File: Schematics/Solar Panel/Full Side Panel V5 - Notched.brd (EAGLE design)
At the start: 50 x 50 mm, 24 parts

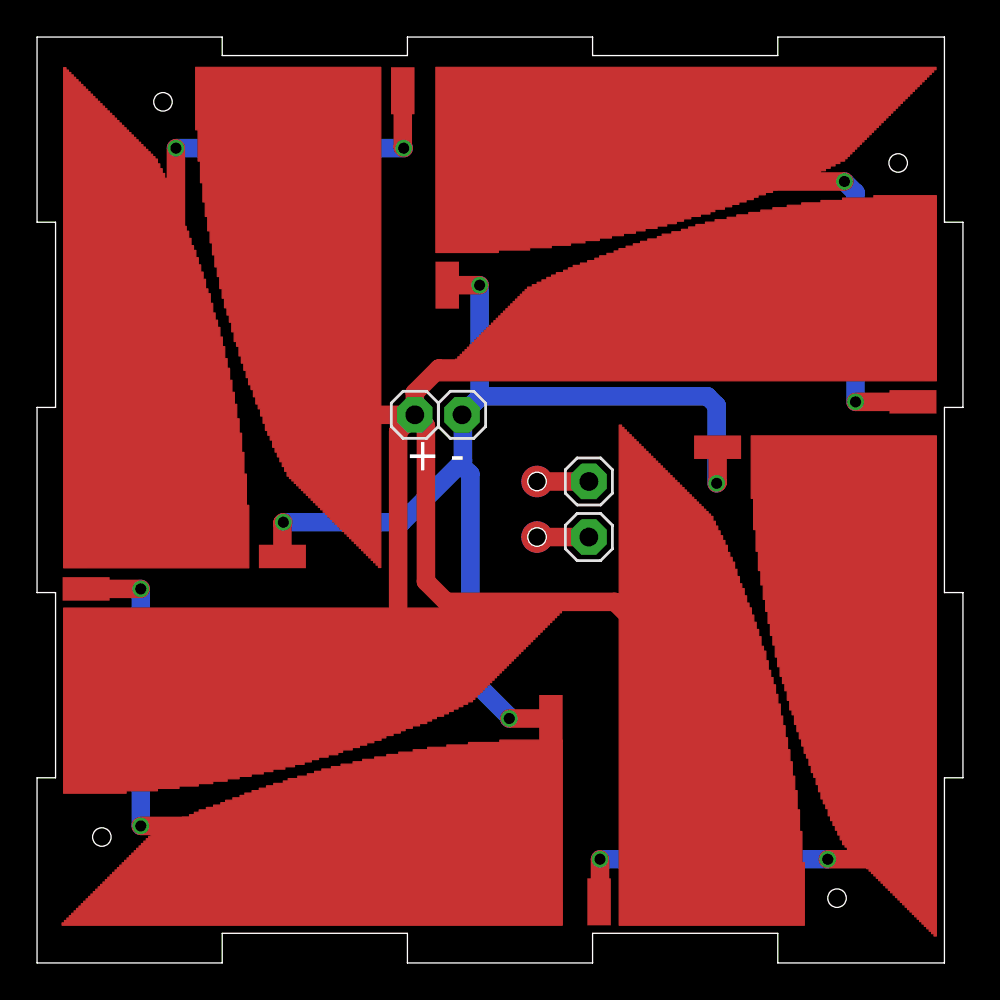
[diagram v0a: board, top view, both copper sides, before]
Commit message: many changes
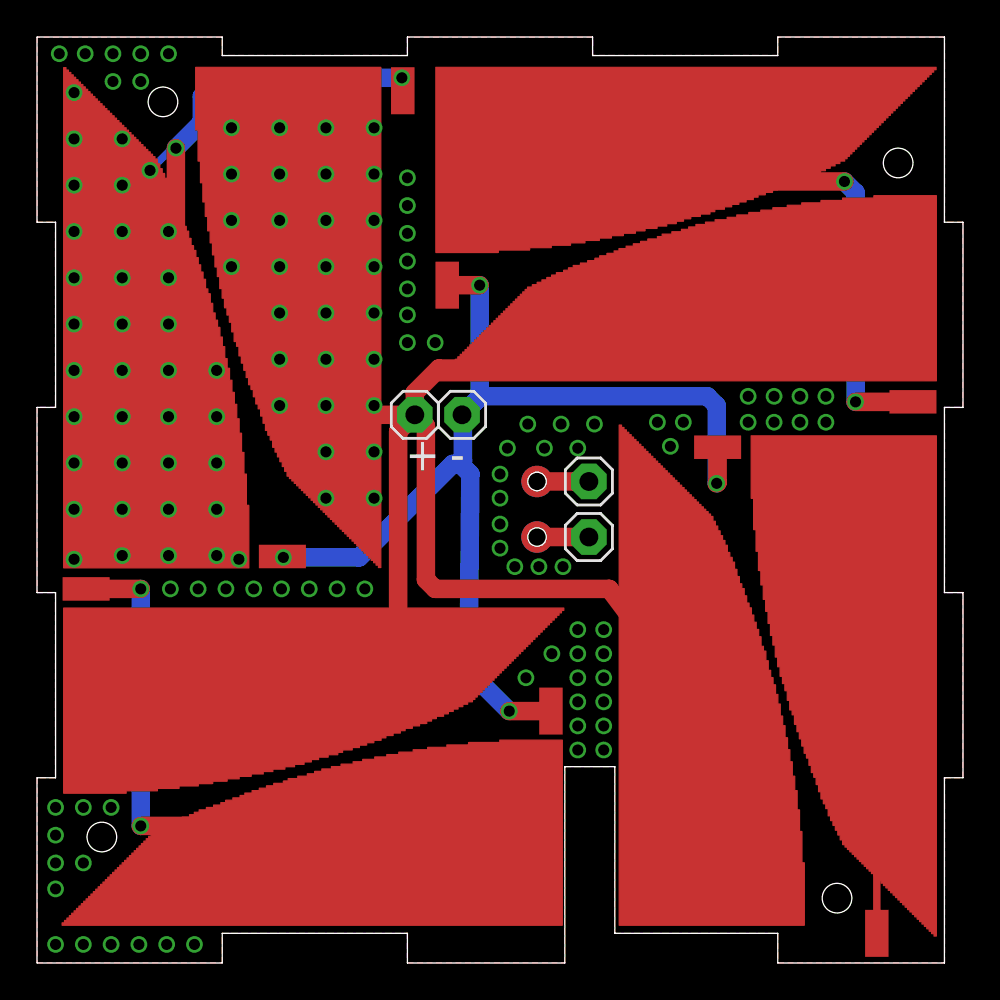
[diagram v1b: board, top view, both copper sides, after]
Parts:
- moved E$15 15.1 mm to (45.4, 1.60)
- moved E$12 0.40 mm to (27.8, 13.6)
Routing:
- net S$2: track 42.4 -> 29.1 mm, vias 2 -> 0
- net S$4: track 40.0 -> 42.3 mm, vias 2 -> 38
- net GND: track 62.2 -> 60.9 mm
- added copper zone on layer 1, net S$10
- added copper zone on layer 16, net S$13
- added copper zone on layer 16, net S$4
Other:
- outline, holes or cut-outs redrawn
